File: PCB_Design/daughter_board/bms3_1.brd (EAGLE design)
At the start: 116.9 x 114.3 mm, 160 parts, among them T1 RTR020P02, T10 RTR020P02, T11 RTR020P02, T12 RTR020P02, T2 RTR020P02, T3 RTR020P02, T4 RTR020P02, T5 RTR020P02, T6 RTR020P02, T7 RTR020P02, T8 RTR020P02, T9 RTR020P02

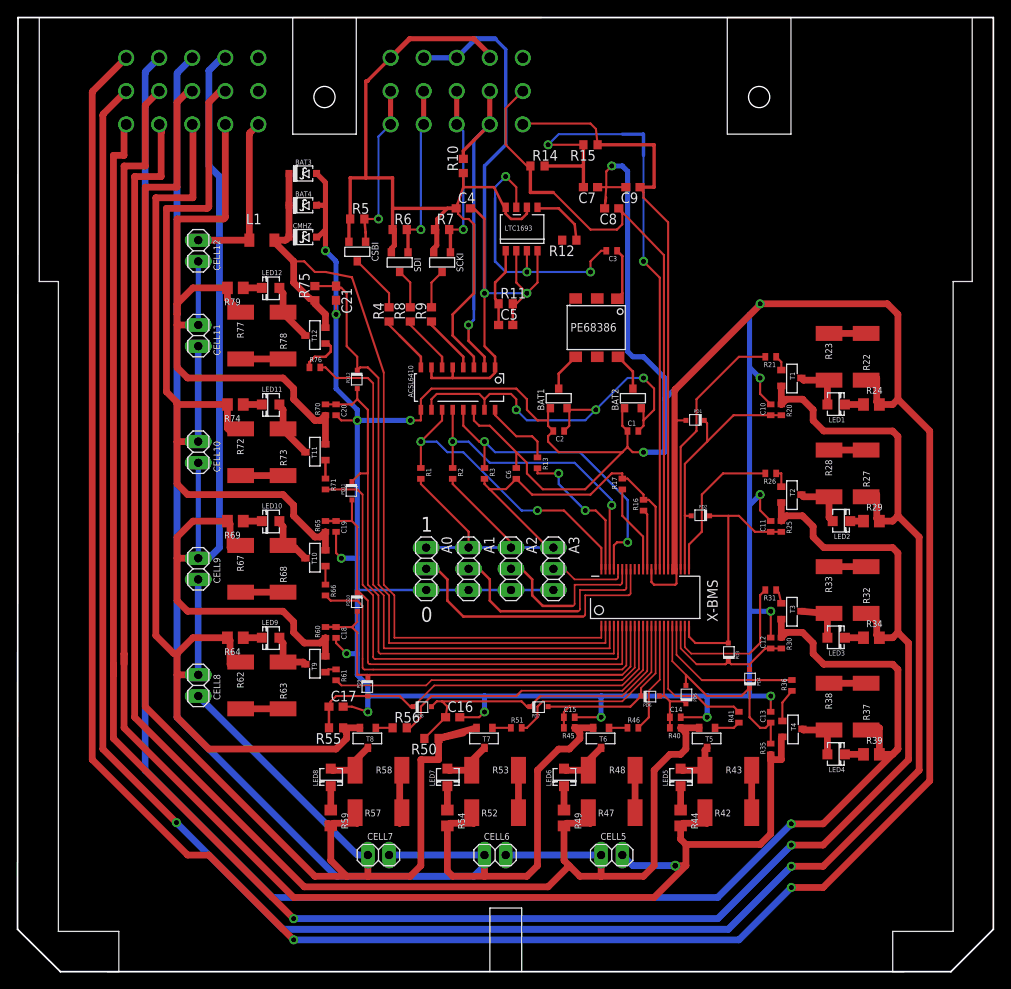
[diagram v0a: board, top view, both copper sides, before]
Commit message: more 0603
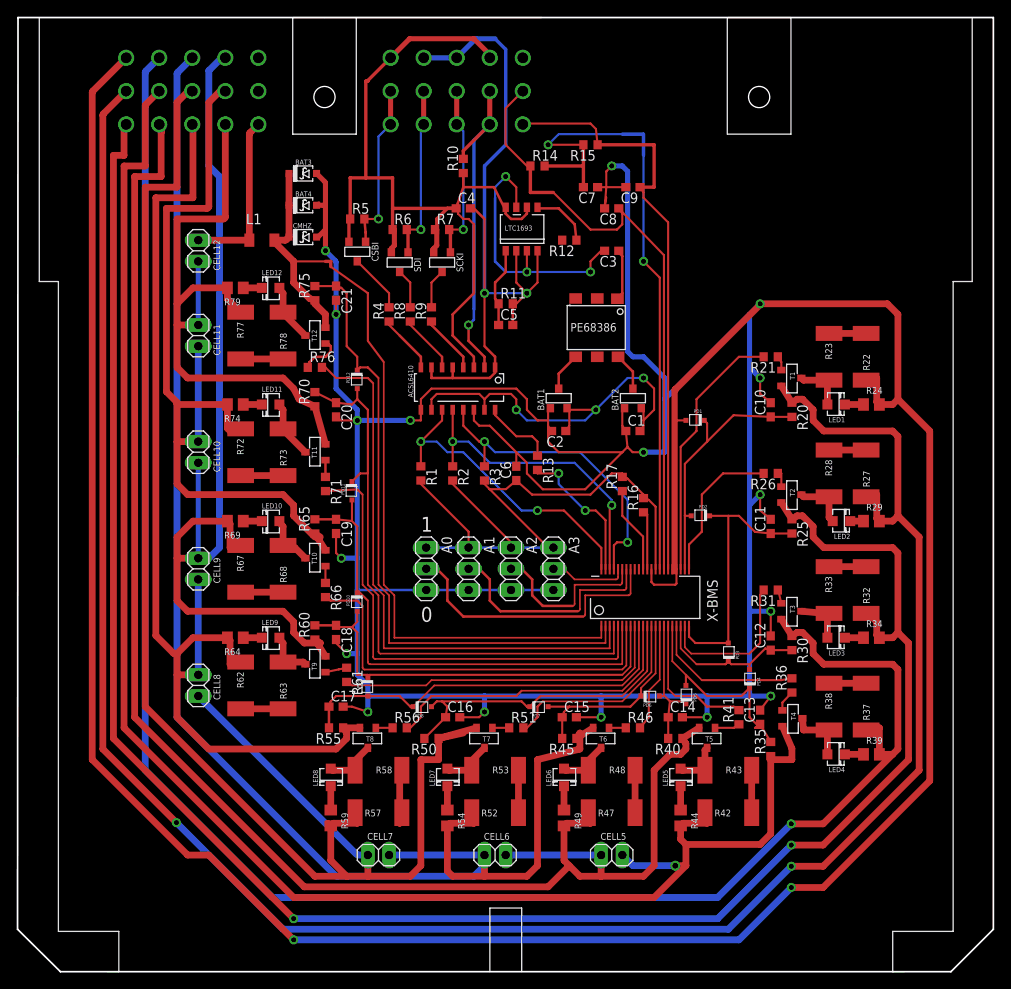
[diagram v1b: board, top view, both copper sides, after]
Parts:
- C1, C10, C11, C12, C13, C14, C15, C18, C19, C2, C20, C3, C6: device rcl:C0402 -> rcl:C0603
- R1, R13, R16, R17, R2, R20, R21, R25, R26, R3, R30, R31, R35, R36, R40, R41, R45, R46, R51, R60, R61, R65, R66, R70, R71, R76: device rcl:R0402 -> rcl:R0603
- moved R70 1.80 mm to (35.6, 68.6)
- moved T4 1.27 mm to (91.6, 30.4)
- moved R40 1.27 mm to (78.7, 27.9)
- moved R45 1.27 mm to (66.0, 27.9)
- moved C13 1.27 mm to (88.9, 30.5)
- moved R20 1.27 mm to (92.7, 67.3)
- moved R25 1.27 mm to (92.7, 53.3)
- moved R30 1.27 mm to (92.7, 39.4)
- moved R60 1.27 mm to (35.6, 40.6)
- moved R61 1.27 mm to (39.4, 35.6)
- moved R65 1.27 mm to (35.6, 53.3)
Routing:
- net CELL11: track 81.5 -> 78.5 mm
- net CELL2: track 238.8 -> 236.3 mm
- net CELL3: track 225.9 -> 223.8 mm
- net CELL0: track 714.2 -> 712.5 mm
- net C11FILTER: track 70.5 -> 72.1 mm
- net C9FILTER: track 49.9 -> 51.3 mm
- net T4: track 4.02 -> 2.60 mm
- net DC9: track 41.9 -> 40.5 mm
- net C6FILTER: track 23.6 -> 24.9 mm
- net C3FILTER: track 17.2 -> 18.5 mm
- net C10FILTER: track 58.7 -> 60.0 mm
- net C5FILTER: track 15.1 -> 16.4 mm
- net C2FILTER: track 30.9 -> 32.2 mm
- net C1FILTER: track 30.0 -> 31.3 mm
- net CELL1: track 261.8 -> 260.6 mm
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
